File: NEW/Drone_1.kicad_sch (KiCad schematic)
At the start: 29 parts, among them J1 ESP-32_DevkitC, J2 Conn_01x08_Pin, U1 Rasberry Pi 0W, U2 MPU6050, U3 GY-NEO6MV2, U4 BME280, U5 HMC5883L, U6 mp1584, U7 mp1584, U8 Flysky fs-a8s

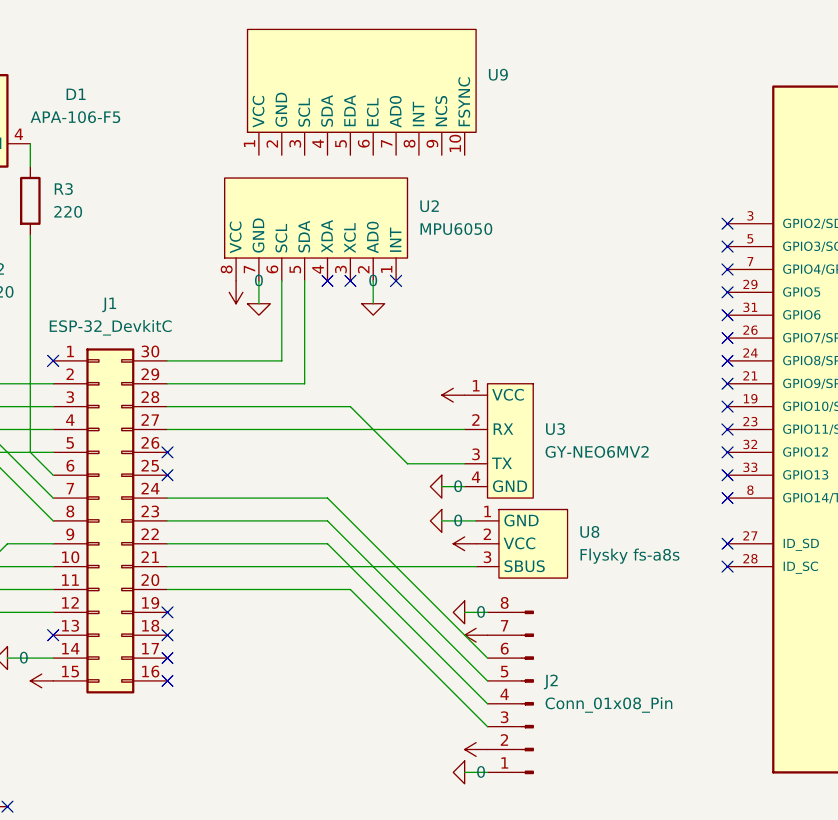
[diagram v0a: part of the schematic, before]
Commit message: welcome
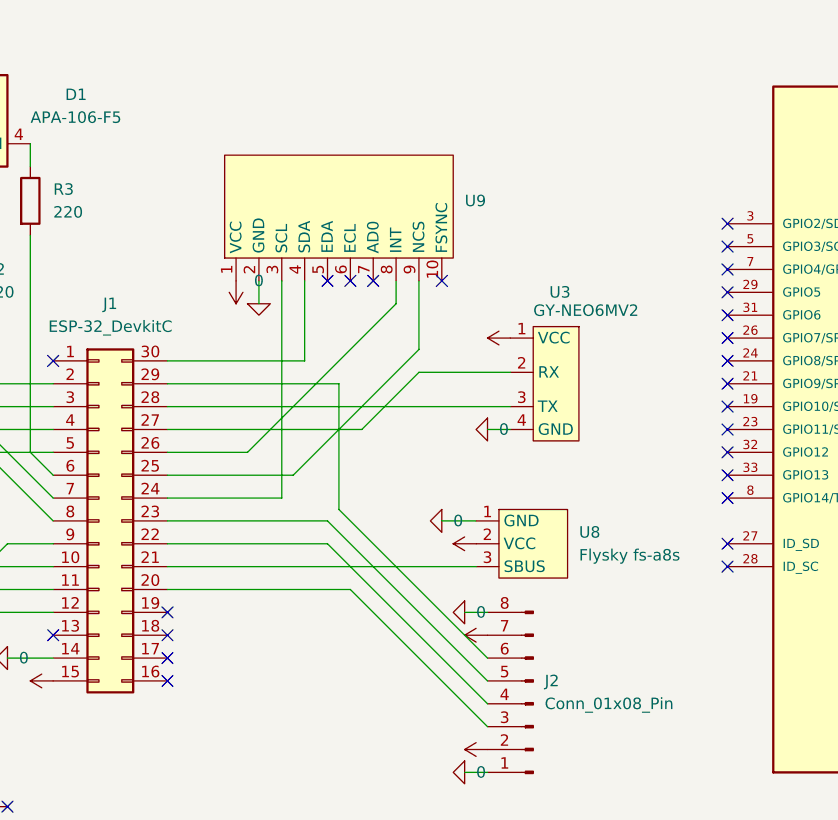
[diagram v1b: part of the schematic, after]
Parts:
- removed U2: MPU6050, MPU6050_footprint:MPU6050foot, symbol MPU6050_module:MPU6050m
- U9: footprint (none) -> MPU6500:MPU6500
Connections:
- net +3.3V: now also U9.1 (VCC)
- net 0: now also U9.2 (GND)
- net at J1.29 (Pin_29): now also J2.6 (Pin_6)
- net at J1.30 (Pin_30): now also U9.4 (SDA)
- net at J1.24 (Pin_24): now also U9.3 (SCL); no longer J2.6 (Pin_6)
- net at U9.8 (INT): now also J1.26 (Pin_26)
- net at U9.9 (NCS): now also J1.25 (Pin_25)
- no-connect marks 64 -> 63
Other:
- moved on the sheet: U3, U9
